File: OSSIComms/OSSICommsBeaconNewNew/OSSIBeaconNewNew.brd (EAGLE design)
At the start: 94 x 88 mm, 77 parts, among them Q1 NX-3215, U1 OPA2347, U2 MSP430F2132, U3 LM7321, U4 MAX1682, U5 MAX890L, U6 MAX4376, U7 TPS3838, U8 MCP1700_SOT23, X1 ESQ-126-38-G-D, X2 5268-03, X3 ICCON_POWERCON, X4 ICCON_POWERCON, X5 WEIDMULLER, X6 JTAG10PINMINI-H, X7 5268-03

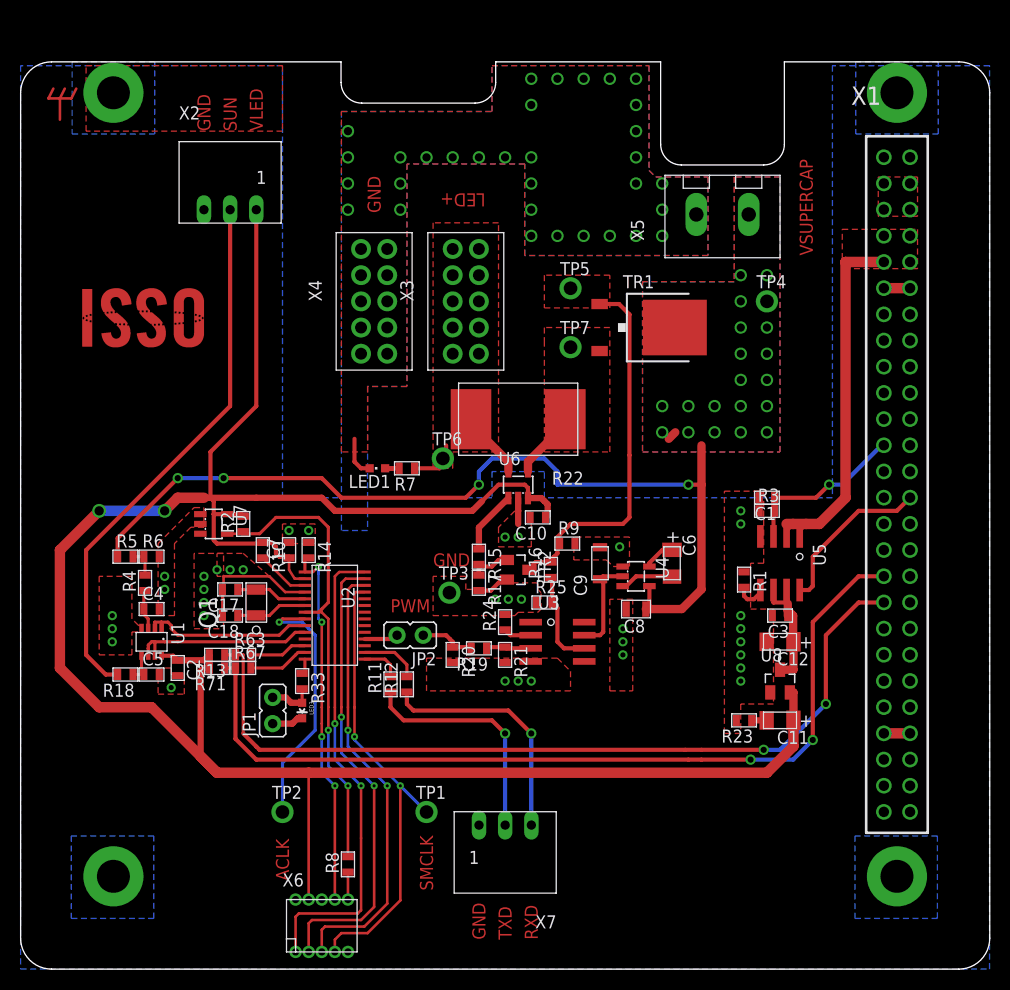
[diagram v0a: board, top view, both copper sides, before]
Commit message: beacon newnew led new
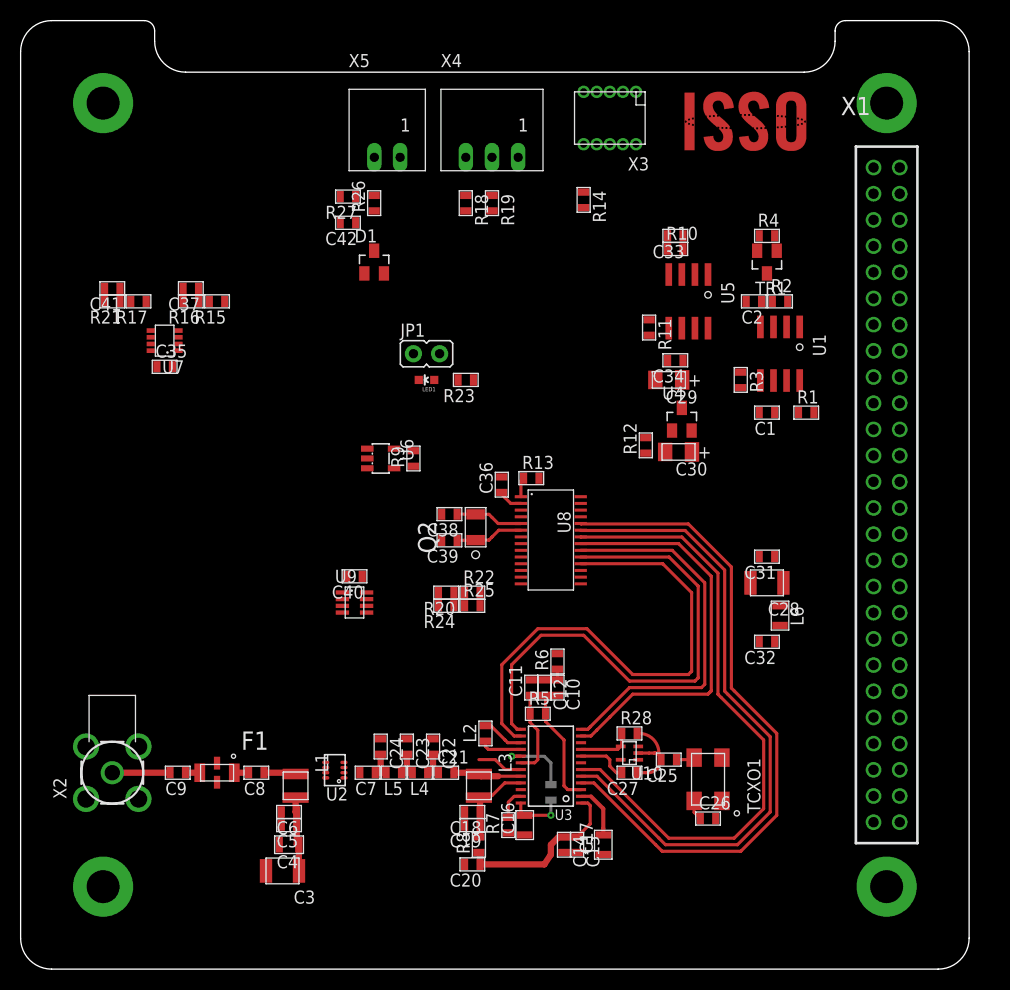
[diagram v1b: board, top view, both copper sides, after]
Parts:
- removed JP2: (no value), OSSI:JP1
- removed LED3: (no value), SparkFun:LED-0603
- removed Q1: NX-3215, OSSI:NX-3215
- removed R33: 1k, OSSI:R0603(1608)
- removed R63, R67: 250, OSSI:R0603(1608)
- removed R71: 10k, OSSI:R0603(1608)
- removed TP1, TP2, TP3, TP4, TP5, TP6, TP7: TP, OSSI:TP-13
- removed TR2: FDV301N, OSSI:SOT23
- removed X6: JTAG10PINMINI-H, OSSI:M50-3200545
- removed X7: 5268-03, OSSI:5268-03
- added C13: 22nF, OSSI:C0603(1608)
- added C14: 1uF,0603, OSSI:C0603(1608)
- added C15: 100pF, OSSI:C0603(1608)
- added C16: 1uF 0805, OSSI:C0805(2012)
- added C19, C33: 1uF, OSSI:C0603(1608)
- added C20: (no value), OSSI:C0603(1608)
- added C21, C25: 1nF, OSSI:C0603(1608)
- added C22, C23, C24: 22pF, OSSI:C0603(1608)
- added C26, C31: 10nF, OSSI:C0603(1608)
- added C27: DNP, OSSI:C0603(1608)
- added C28: 22uF,1210, OSSI:C1210-GCM32
- added C29, C30: 10uF, LDO Tantal 16V, OSSI:C1206(3216)-A
- added C32, C34, C35, C36, C40, C42: 100nF, OSSI:C0603(1608)
- added C37, C41: TBD, OSSI:C0603(1608)
- added C38, C39: 12.5pF, OSSI:C0603(1608)
- added D1: BAT54S, OSSI:SOT23
- added F1: LFCN-160, OSSI:LFCN
- added L1, L3: 470nH, 1008 size, OSSI:L1008(2520)
- added L2: 10nH, OSSI:L0603(1608)
- added L4, L5: 68nH, OSSI:L0603(1608)
- added L6: 5~15R ferrite bead, OSSI:L0805(2012)
- added Q2: NX-3215, OSSI:NX-3215
- added R26: 4.7k, OSSI:R0603(1608)
- added R27: 47k, OSSI:R0603(1608)
- added R28: 1M, OSSI:R0603(1608)
- added TCXO1: 19.2MHz, OSSI:TCXO_M532
- added U10: NC7SZ04, OSSI:SC70-5
- added U9: MAX6369, OSSI:SOT23-8
- C1: value 1uF -> 100nF
- C10: value 100nF -> 1000pF
- C11: value 10uF, LDO Tantal 16V -> 22pF; device OSSI:C1206(3216)-A -> OSSI:C0603(1608)
- C12: value 10uF, LDO Tantal 16V -> 68pF; device OSSI:C1206(3216)-A -> OSSI:C0603(1608)
- C17: value 12.5pF -> 2.2uF, 0805; device OSSI:C0603(1608) -> OSSI:C0805(2012)
- C18: value 12.5pF -> 100pF
- C2: value 100nF -> 1uF
- C3: value 100nF -> 22uF,1210; device OSSI:C0603(1608) -> OSSI:C1210-GCM32
- C4: value 100nF -> 1uF,0805; device OSSI:C0603(1608) -> OSSI:C0805(2012)
- C6: value 10uF, LDO Tantal 16V -> 10nF; device OSSI:C1206(3216)-A -> OSSI:C0603(1608)
- C7: value 100nF -> 10nF
- C8: value 1uF 0805 -> 10nF; device OSSI:C0805(2012) -> OSSI:C0603(1608)
- C9: value 1206 Cap -> (none); device OSSI:C1206-GCM31 -> OSSI:C0603(1608)
- LED1: device led:CHIPLED_0603 -> SparkFun:LED-0603
- R1, R10: value TBD -> 100k
- R11: value 4.7k -> 23.7k
- R12, R8: value 4.7k -> 0
- R13: value 10k -> 4.7k
- R14: value 47k -> 4.7k
- R15, R17, R21: value (none) -> 100k
- R18: value 1k -> 4.7k
- R19: value (none) -> 4.7k
- R20: value (none) -> 10k
- R22: value 0.005, 2W RSENSE -> 250; device OSSI:R4527(12070) -> OSSI:R0603(1608)
- R23: value 0 -> 1k
- R24: value 1.1k -> 10k
- R25: value 2.2k -> 250
- R3: value 100k -> 6.2k
- R4: value 1k -> 100k
- R5: value 100k -> 5.1k
- R6: value 100k -> 2.4k
- R7: value 1.5k -> 3.6k
- R9: value DNP -> 100k
- TR1: value FDD8896 -> FDV301N; device OSSI:TO252 -> OSSI:SOT23
- U1: value OPA2347 -> MAX890L; device OSSI:SOT23-8DCN -> OSSI:SO8
- U2: value MSP430F2132 -> ADL5530; device OSSI:PW28 -> OSSI:LFCSP8_CP
- U3: value LM7321 -> ADF7012; device OSSI:SO8 -> OSSI:TSSOP24
- U4: value MAX1682 -> MCP1700_SOT23; device OSSI:SOT23-5DBV -> OSSI:SOT23
- U6: value MAX4376 -> TPS3838
- U7: value TPS3838 -> OPA2347; device OSSI:SOT23-5DBV -> OSSI:SOT23-8DCN
- U8: value MCP1700_SOT23 -> MSP430F2132; device OSSI:SOT23 -> OSSI:PW28
- X2: value 5268-03 -> RFCON-MCX-R/A; device OSSI:5268-03 -> OSSI:MCX-R/A
- X3: value ICCON_POWERCON -> JTAG10PINMINI-H; device OSSI:ICCON6643220-1 -> OSSI:M50-3200545
- X4: value ICCON_POWERCON -> 5268-03; device OSSI:ICCON6643220-1 -> OSSI:5268-03
- X5: value WEIDMULLER -> 5268-02; device OSSI:WEIDMULLER1760490000 -> OSSI:5628-02
- moved R4 69.1 mm to (72.4, 71.1), turned to 0 degrees
- moved U1 67.1 mm to (73.7, 59.7)
- moved C2 66.2 mm to (71.1, 64.8), turned to 180 degrees
- moved U$1 61.4 mm to (76.2, 85.1)
- moved R18 56.4 mm to (43.2, 74.3), turned to 270 degrees
- moved R2 56.4 mm to (73.7, 64.8), turned to 0 degrees
- moved X2 55.8 mm to (8.89, 19.1), turned to 90 degrees
- moved C3 54.2 mm to (25.4, 9.53)
- moved R21 51.3 mm to (8.89, 64.8), turned to 180 degrees
- moved R10 49.5 mm to (63.5, 69.8), turned to 0 degrees
- moved C9 45.7 mm to (15.2, 19.1), turned to 180 degrees
- moved C6 44.3 mm to (26.0, 15.2), turned to 180 degrees
- moved C17 43.9 mm to (56.5, 12.1), turned to 90 degrees
- moved R16 43.6 mm to (16.5, 64.8), turned to 180 degrees
- moved R19 43.2 mm to (45.7, 74.3), turned to 270 degrees
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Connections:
- removed net 3.3VLED: C10.1, C11.1, C2.1, C7.1, R10.1, R13.2, R2.2, R71.2, U1.8, U2.2, U6.3, U7.5, U8.2, X2.1, X6.4
- removed net ACLK_OUT: TP2.TP, U2.8
- removed net ADC2: U1.6, U1.7, U2.10
- removed net PWM: JP2.1, R19.2, R20.1
- removed net RESET_LED: R2.1, R8.2, U2.7, U7.4
- removed net SMCLK_OUT: TP1.TP, U2.25, X6.7
- removed net STRUT_GND: H1.B3,2
- removed net SUN: R18.2, X2.2
- new net 3.3VBEACON: C28.P$1, C30.1, C31.1, C35.1, C36.1, D1.2, L6.1, R1.2, R20.2, R24.2, R9.2, U4.2, U6.5, U7.8, U8.2, U9.4, U9.5, U9.6, U9.8, X3.4, X5.1
- new net ADC0: U7.6, U7.7, U8.8
- new net BEACON_CE: U3.14, U8.18
- new net BEACON_CWCONTROL: R26.2, R27.1, X5.2
- new net BEACON_DATA: U3.4, U8.24
- new net BEACON_MUXOUT: U3.6, U8.22
- new net BEACON_RFOUT: C24.2, C7.1, L5.2
- new net BEACON_SCLK: U3.11, U8.21
- new net BEACON_SDATA: U3.12, U8.20
- new net BEACON_SLE: U3.13, U8.19
- new net BEACON_TXCLK: U3.5, U8.23
- new net BEACON_WDT_RST: C40.1, U6.3, U9.7
- new net N$1: R23.1, U8.11
- new net N$2: U8.27, X3.3
- new net N$34: C8.2, F1.1
- new net N$35: C9.1, F1.3
- new net N$36: C23.2, L4.2, L5.1
- new net N$37: C9.2, X2.1
- new net N$38: C25.2, C27.1, R28.2, U10.2
- new net N$40: C30.2, R12.1
- new net N$666: C29.1, C34.1, U4.3, U5.6, U5.7
- new net N$69: C25.1, TCXO1.3
- new net OSC1: C27.2, U3.8
- new net OSC2: R28.1, U10.4, U3.9
- new net PA_-FAULT: R1.1, U1.8, U8.3
- new net PA_ON: R4.2, TR1.1, U8.17
- new net RESETBEACON: R14.2, R9.1, U6.4, U8.7
- new net VBEACON_PA: C1.1, C3.P$1, C4.1, C5.1, C6.1, L1.P$1, U1.6, U1.7
- new net VCCRF: C14.1, C15.1, C20.1, C26.1, C32.1, L6.2, R8.1, TCXO1.4, U10.5, U3.1
- net ADC1: now also U7.1, U7.2, U8.9; no longer U1.1, U1.2, U2.9
- net BEACON_-FAULT: now also U5.8
- net BEACON_OFF: now also C33.1, R10.2, U5.3
- net BEACON_SCL: now also R24.1, R25.1
- net BEACON_SDA: now also R20.1, R22.1
- net BUS_CS: now also R15.1
- net GND: now also C11.2, C12.1, C14.2, C15.2, C16.1, C17.1, C19.2, C20.2, C22.1, C23.1, C24.1, C26.2, C28.P$2, C29.2, C3.P$2, C31.2, C32.2, C33.2, C34.2, C35.2, C36.2, C37.2, C38.2, C39.2, C40.2, C41.2, C42.2, C6.2, D1.1, F1.2, F1.4, R10.1, R11.1, R12.2, R13.2, R16.2, R27.2, R4.1, R7.1, TCXO1.1, TCXO1.2, TR1.2, U10.3, U2.1, U2.3, U2.5, U2.6, U2.8, U3.19, U3.22, U3.7, U6.1, U7.4, U8.4, U9.2, X2.2, X2.4, X2.5, X3.9; no longer C10.2, C12.2, C17.2, C3.2, C7.2, C8.2, C9.P$2, LED3.C, R1.1, R14.1, R17.2, R20.2, R23.2, R24.2, R25.1, R9.2, TP3.TP, TR2.2, U3.4, U7.1, U7.2, U8.1, X4.10, X4.2, X4.3, X4.4, X4.5, X4.6, X4.7, X4.8, X4.9, X5.2, X6.9, X7.1
- net LED_-FAULT: no longer U5.8
- net LED_OFF: no longer C1.1, R3.2, U5.3
- net LED_SCL: no longer R67.1, R71.1
- net LED_SDA: no longer R13.1, R63.1
- net N$10: now also R25.2, U8.13; no longer R1.2, U5.5
- net N$11: now also R18.2, U8.16; no longer R4.2, R5.2, R6.1
- net N$12: now also U8.10, U9.1; no longer R22.P$2, R7.1, TP6.TP, U6.5, X3.1, X3.10, X3.2, X3.3, X3.4, X3.5, X3.6, X3.7, X3.8, X3.9
- net N$13: now also C42.1, D1.3, R26.1, U8.14; no longer C9.P$1, U3.7, U4.2
- net N$14: now also L2.1, U3.16; no longer R16.1, R25.2, U3.6
- net N$15: now also L2.2, U3.15; no longer U2.27, X6.3
- net N$16: now also C13.1, C16.2, U3.24; no longer R22.P$1, TP7.TP, TR1.S, U6.4
- net N$17: now also C13.2, U3.17; no longer C11.2, R23.1
- net N$18: now also R7.2, U3.23; no longer R24.1, U3.2
- net N$19: now also C2.1, R2.1, TR1.3, U1.3; no longer C17.1, Q1.2, U2.5
- net N$20: now also C10.1, R6.1; no longer C18.1, Q1.1, U2.6
- net N$21: now also R3.2, U1.5; no longer JP1.2, LED3.A, R33.2
- net N$22: now also C41.1, R17.2, R21.1, U7.5; no longer R63.2, U2.12
- net N$23: now also C21.2, L3.P$2, U3.20; no longer R67.2, U2.13
- net N$24: now also C11.1, R5.1, U3.18; no longer R15.1, U6.1
- net N$25: now also C17.2, U3.2; no longer R33.1, U2.14
- net N$26: now also C10.2, C12.2, R5.2, U3.3; no longer C6.2, U4.3
- net N$27: now also C18.1, C19.1, L3.P$1, R8.2, U3.21; no longer C6.1, U4.5
- net N$28: now also C7.2, U2.2; no longer R12.2, U2.16
- net N$29: now also C21.1, C22.2, L4.1; no longer LED1.A, R7.2
- net N$3: now also U8.26, X3.5; no longer U2.28, X6.1
- net N$30: now also C8.1, L1.P$2, U2.7; no longer R15.2, R17.1, TR2.1
- net N$31: now also R14.1, X3.10; no longer U2.26, X6.5
- net N$32: now also R11.2, U5.5; no longer R8.1, X6.10
- net N$33: now also C37.1, R15.2, R16.1, U7.3; no longer JP2.2, U2.18
- net N$39: now also R19.2, U8.15; no longer R11.2, U2.15
- net N$4: now also U8.25, X3.7; no longer R10.2, U2.3
- net N$5: now also C38.1, Q2.2, U8.5; no longer C12.1, C3.1, U5.6, U5.7, U8.3
- net N$6: now also C39.1, Q2.1, U8.6; no longer R16.2, R9.1, TP5.TP, TR1.G, TR2.3
- net N$7: now also JP1.2, LED1.A, R23.2; no longer C4.1, R4.1, U1.3
- net N$8: now also U8.28, X3.1; no longer C5.1, R18.1, U1.5
- net N$9: now also R22.2, U8.12; no longer R19.1, R21.1, U3.3
- net RXD: now also R18.1, X4.3; no longer R12.1, X7.3
- net TEST: now also R13.1, U8.1, X3.8; no longer R14.2, U2.1, X6.8
- net TXD: now also R19.1, X4.2; no longer R11.1, X7.2
- net VBUS: now also R17.1, R2.2, U1.1, U1.2
- net VSUPERCAP: now also X1.13; no longer C8.1, R5.1, TP4.TP, TR1.D, U4.4, X5.1
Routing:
- net 3.3VLED: track 226.5 -> 0.00 mm, vias 2 -> 0
- net VSUPERCAP: track 89.2 -> 0.00 mm, vias 23 -> 0
- net LED_SCL: track 85.9 -> 0.00 mm, vias 2 -> 0
- net LED_SDA: track 82.0 -> 0.00 mm, vias 2 -> 0
- net BEACON_DATA: track 0.00 -> 65.5 mm
- net BEACON_TXCLK: track 0.00 -> 63.3 mm
- net BEACON_MUXOUT: track 0.00 -> 61.1 mm
- net SUN: track 52.8 -> 0.00 mm
- net BEACON_SLE: track 0.00 -> 49.5 mm
- net BEACON_CE: track 0.00 -> 49.4 mm
- net N$3: track 46.7 -> 0.00 mm, vias 2 -> 0
- net RESET_LED: track 46.2 -> 0.00 mm, vias 2 -> 0
- net SMCLK_OUT: track 45.4 -> 0.00 mm, vias 2 -> 0
- net N$31: track 43.4 -> 0.00 mm, vias 2 -> 0
- net N$15: track 45.0 -> 4.12 mm, vias 2 -> 0
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- removed copper zone on layer 1, net GND
- removed copper zone on layer 16, net GND
- removed copper zone on layer 16, net N$1
- removed copper zone on layer 1, net N$12
- removed copper zone on layer 1, net N$16
- removed copper zone on layer 16, net N$2
- removed copper zone on layer 16, net N$56
- removed copper zone on layer 1, net N$6
- removed copper zone on layer 1, net STRUT_GND
- removed copper zone on layer 1, net VBUS
- removed copper zone on layer 1, net VSOLAR
- removed copper zone on layer 1, net VSUPERCAP
- removed copper zone on layer 16, net VSUPERCAP
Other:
- board size 94 x 88 mm -> 92 x 92 mm
- board text removed: "ACLK"
- board text removed: "GND"
- board text removed: "LED+"
- board text removed: "PWM"
- board text removed: "RXD"
- board text removed: "SMCLK"
- board text removed: "SUN"
- board text removed: "TXD"
- board text removed: "VLED"
- board text removed: "VSUPERCAP"
